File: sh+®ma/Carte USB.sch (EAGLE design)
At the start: 12 parts, among them X2 PN61729-S, X4 87758-0216, X5 PN61729-S, X7 PN61729-S, X8 PN61729-S

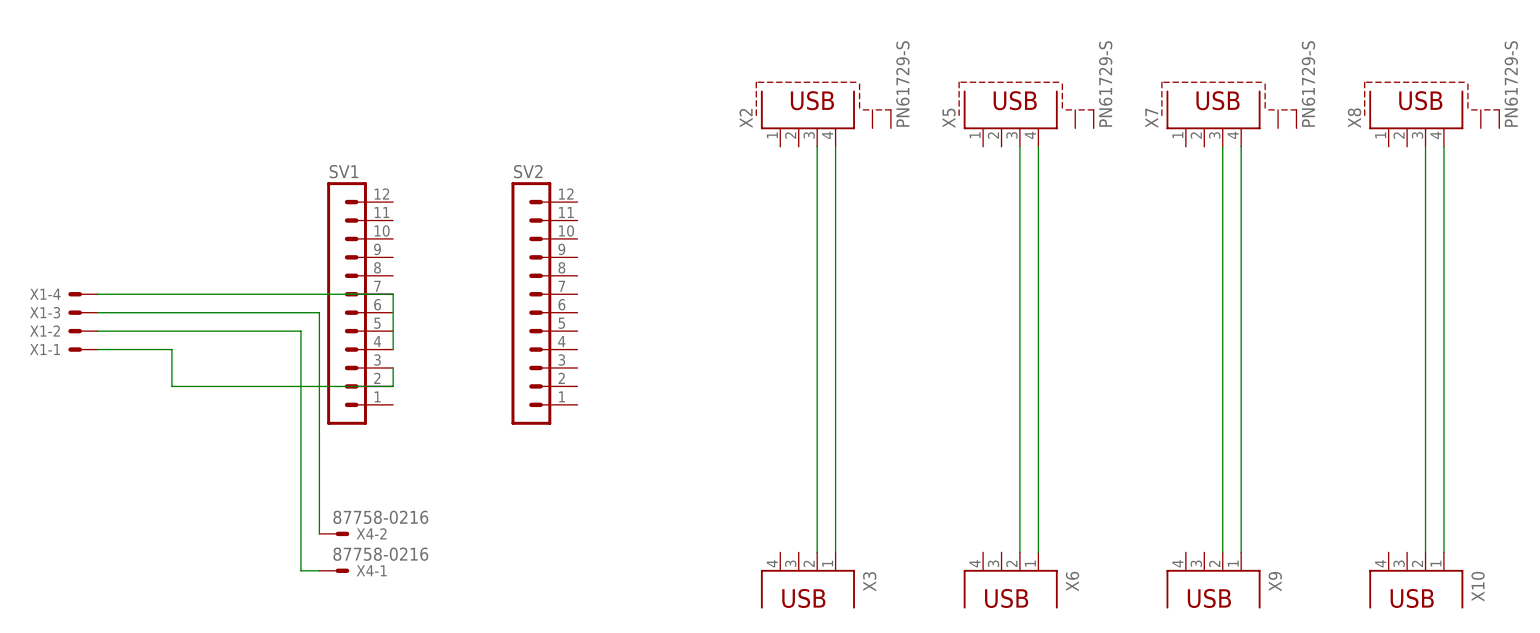
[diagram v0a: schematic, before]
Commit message: typon + plaque fond
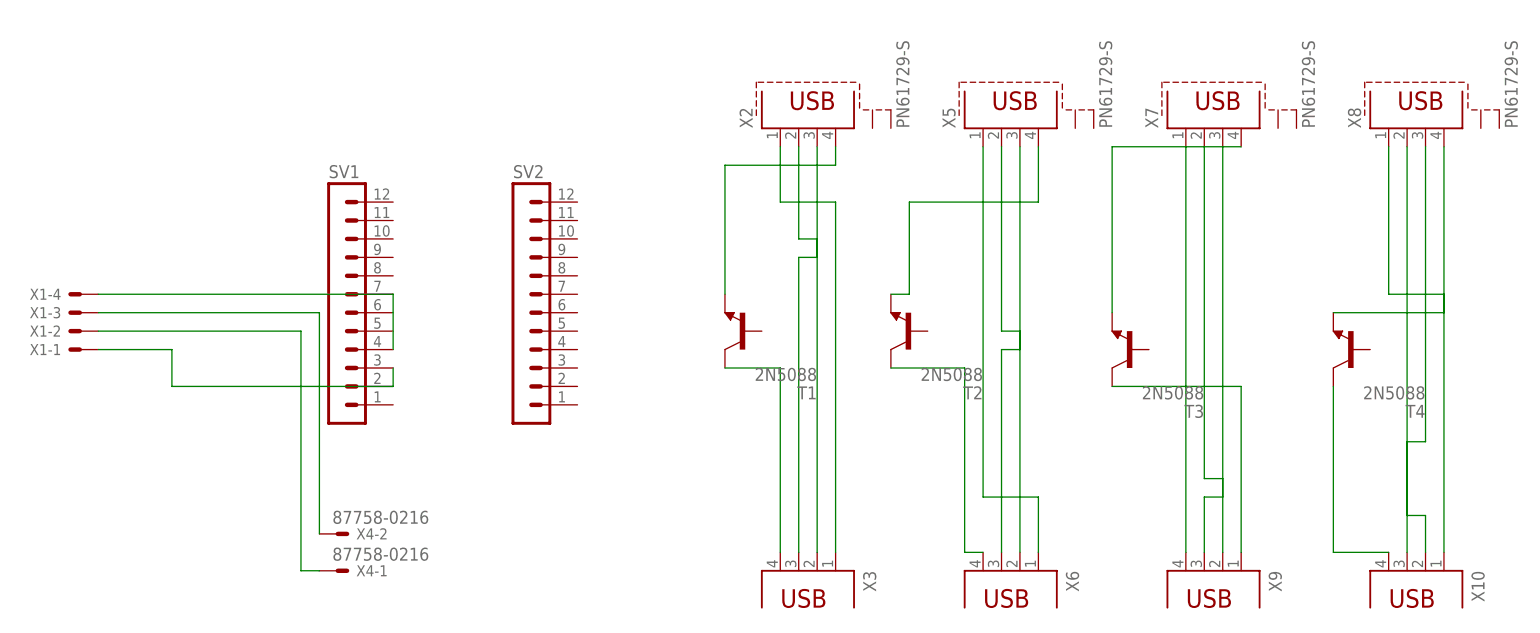
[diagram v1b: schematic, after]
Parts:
- added T1, T2, T3, T4: 2N5088, transistor:2N5088
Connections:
- new net N$14: X7.3, X9.3
- new net N$15: X10.1, X8.1
- new net N$16: X10.2, X8.2
- new net N$17: X10.3, X8.3
- new net N$18: T1.E, X2.4
- new net N$19: T1.C, X3.4
- new net N$20: T2.C, X6.4
- new net N$21: T2.E, X5.4
- new net N$22: T3.E, X7.4
- new net N$23: T3.C, X9.4
- new net N$24: T4.C, X10.4
- new net N$25: T4.E, X8.4
- net N$10: now also X5.2, X6.2; no longer X7.4, X9.1
- net N$11: now also X7.1, X9.1; no longer X10.2, X8.3
- net N$12: now also X7.2, X9.2; no longer X10.1, X8.4
- net N$3: now also X2.1; no longer X2.4
- net N$4: now also X2.2; no longer X2.3
- net N$7: now also X2.3, X3.3; no longer X5.4, X6.1
- net N$8: now also X6.3; no longer X6.2
- net N$9: now also X5.1, X6.1; no longer X7.3, X9.2
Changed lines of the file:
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@@
 <part name="X9" library="con-berg" deviceset="PN87520" device=""/>
 <part name="X10" library="con-berg" deviceset="PN87520" device=""/>
+<part name="T1" library="transistor" deviceset="2N5088" device=""/>
+<part name="T2" library="transistor" deviceset="2N5088" device=""/>
+<part name="T3" library="transistor" deviceset="2N5088" device=""/>
+<part name="T4" library="transistor" deviceset="2N5088" device=""/>
 </parts>
 <sheets>
@@
 <instance part="X9" gate="G$1" x="144.78" y="15.24" rot="R270"/>
 <instance part="X10" gate="G$1" x="172.72" y="15.24" rot="R270"/>
+<instance part="T1" gate="G$1" x="81.28" y="48.26" rot="R180"/>
+<instance part="T2" gate="G$1" x="104.14" y="48.26" rot="R180"/>
+<instance part="T3" gate="G$1" x="134.62" y="45.72" rot="R180"/>
+<instance part="T4" gate="G$1" x="165.1" y="45.72" rot="R180"/>
 </instances>
 <busses>
@@
 <pinref part="X4" gate="-1" pin="S"/>
 <wire x1="20.32" y1="15.24" x2="22.86" y2="15.24" width="0.1524" layer="91"/>
-</segment>
-</net>
-<net name="N$3" class="0">
-<segment>
-<pinref part="X2" gate="G$1" pin="4"/>
-<pinref part="X3" gate="G$1" pin="1"/>
-<wire x1="93.98" y1="73.66" x2="93.98" y2="17.78" width="0.1524" layer="91"/>
-</segment>
-</net>
-<net name="N$4" class="0">
-<segment>
-<pinref part="X2" gate="G$1" pin="3"/>
-<wire x1="91.44" y1="73.66" x2="91.44" y2="17.78" width="0.1524" layer="91"/>
-<pinref part="X3" gate="G$1" pin="2"/>
 </segment>
 </net>
@@
 </segment>
 </net>
+<net name="N$3" class="0">
+<segment>
+<pinref part="X3" gate="G$1" pin="1"/>
+<wire x1="93.98" y1="17.78" x2="93.98" y2="66.04" width="0.1524" layer="91"/>
+<pinref part="X2" gate="G$1" pin="1"/>
+<wire x1="93.98" y1="66.04" x2="86.36" y2="66.04" width="0.1524" layer="91"/>
+<wire x1="86.36" y1="66.04" x2="86.36" y2="73.66" width="0.1524" layer="91"/>
+</segment>
+</net>
+<net name="N$4" class="0">
+<segment>
+<pinref part="X2" gate="G$1" pin="2"/>
+<wire x1="88.9" y1="73.66" x2="88.9" y2="60.96" width="0.1524" layer="91"/>
+<pinref part="X3" gate="G$1" pin="2"/>
+<wire x1="88.9" y1="60.96" x2="91.44" y2="60.96" width="0.1524" layer="91"/>
+<wire x1="91.44" y1="60.96" x2="91.44" y2="17.78" width="0.1524" layer="91"/>
+</segment>
+</net>
 <net name="N$7" class="0">
 <segment>
+<pinref part="X3" gate="G$1" pin="3"/>
+<wire x1="88.9" y1="17.78" x2="88.9" y2="58.42" width="0.1524" layer="91"/>
+<pinref part="X2" gate="G$1" pin="3"/>
+<wire x1="88.9" y1="58.42" x2="91.44" y2="58.42" width="0.1524" layer="91"/>
+<wire x1="91.44" y1="58.42" x2="91.44" y2="73.66" width="0.1524" layer="91"/>
+</segment>
+</net>
+<net name="N$8" class="0">
+<segment>
+<pinref part="X6" gate="G$1" pin="3"/>
+<wire x1="116.84" y1="17.78" x2="116.84" y2="45.72" width="0.1524" layer="91"/>
+<pinref part="X5" gate="G$1" pin="3"/>
+<wire x1="116.84" y1="45.72" x2="119.38" y2="45.72" width="0.1524" layer="91"/>
+<wire x1="119.38" y1="45.72" x2="119.38" y2="73.66" width="0.1524" layer="91"/>
+</segment>
+</net>
+<net name="N$9" class="0">
+<segment>
+<pinref part="X5" gate="G$1" pin="1"/>
+<wire x1="114.3" y1="73.66" x2="114.3" y2="25.4" width="0.1524" layer="91"/>
+<pinref part="X6" gate="G$1" pin="1"/>
+<wire x1="114.3" y1="25.4" x2="121.92" y2="25.4" width="0.1524" layer="91"/>
+<wire x1="121.92" y1="25.4" x2="121.92" y2="17.78" width="0.1524" layer="91"/>
+</segment>
+</net>
+<net name="N$10" class="0">
+<segment>
+<pinref part="X5" gate="G$1" pin="2"/>
+<wire x1="116.84" y1="73.66" x2="116.84" y2="48.26" width="0.1524" layer="91"/>
+<pinref part="X6" gate="G$1" pin="2"/>
+<wire x1="116.84" y1="48.26" x2="119.38" y2="48.26" width="0.1524" layer="91"/>
+<wire x1="119.38" y1="48.26" x2="119.38" y2="17.78" width="0.1524" layer="91"/>
+</segment>
+</net>
+<net name="N$11" class="0">
+<segment>
+<pinref part="X7" gate="G$1" pin="1"/>
+<wire x1="142.24" y1="73.66" x2="142.24" y2="40.64" width="0.1524" layer="91"/>
+<pinref part="X9" gate="G$1" pin="1"/>
+<wire x1="142.24" y1="40.64" x2="149.86" y2="40.64" width="0.1524" layer="91"/>
+<wire x1="149.86" y1="40.64" x2="149.86" y2="17.78" width="0.1524" layer="91"/>
+</segment>
+</net>
+<net name="N$12" class="0">
+<segment>
+<pinref part="X7" gate="G$1" pin="2"/>
+<wire x1="144.78" y1="73.66" x2="144.78" y2="27.94" width="0.1524" layer="91"/>
+<pinref part="X9" gate="G$1" pin="2"/>
+<wire x1="144.78" y1="27.94" x2="147.32" y2="27.94" width="0.1524" layer="91"/>
+<wire x1="147.32" y1="27.94" x2="147.32" y2="17.78" width="0.1524" layer="91"/>
+</segment>
+</net>
+<net name="N$14" class="0">
+<segment>
+<pinref part="X9" gate="G$1" pin="3"/>
+<wire x1="144.78" y1="17.78" x2="144.78" y2="25.4" width="0.1524" layer="91"/>
+<pinref part="X7" gate="G$1" pin="3"/>
+<wire x1="144.78" y1="25.4" x2="147.32" y2="25.4" width="0.1524" layer="91"/>
+<wire x1="147.32" y1="25.4" x2="147.32" y2="73.66" width="0.1524" layer="91"/>
+</segment>
+</net>
+<net name="N$15" class="0">
+<segment>
+<pinref part="X10" gate="G$1" pin="1"/>
+<wire x1="177.8" y1="17.78" x2="177.8" y2="53.34" width="0.1524" layer="91"/>
+<pinref part="X8" gate="G$1" pin="1"/>
+<wire x1="177.8" y1="53.34" x2="170.18" y2="53.34" width="0.1524" layer="91"/>
+<wire x1="170.18" y1="53.34" x2="170.18" y2="73.66" width="0.1524" layer="91"/>
+</segment>
+</net>
+<net name="N$16" class="0">
+<segment>
+<pinref part="X8" gate="G$1" pin="2"/>
+<wire x1="172.72" y1="73.66" x2="172.72" y2="22.86" width="0.1524" layer="91"/>
+<pinref part="X10" gate="G$1" pin="2"/>
+<wire x1="172.72" y1="22.86" x2="175.26" y2="22.86" width="0.1524" layer="91"/>
+<wire x1="175.26" y1="22.86" x2="175.26" y2="17.78" width="0.1524" layer="91"/>
+</segment>
+</net>
+<net name="N$17" class="0">
+<segment>
+<pinref part="X8" gate="G$1" pin="3"/>
+<wire x1="175.26" y1="73.66" x2="175.26" y2="33.02" width="0.1524" layer="91"/>
+<pinref part="X10" gate="G$1" pin="3"/>
+<wire x1="175.26" y1="33.02" x2="172.72" y2="33.02" width="0.1524" layer="91"/>
+<wire x1="172.72" y1="33.02" x2="172.72" y2="17.78" width="0.1524" layer="91"/>
+</segment>
+</net>
+<net name="N$18" class="0">
+<segment>
+<pinref part="X2" gate="G$1" pin="4"/>
+<wire x1="93.98" y1="73.66" x2="93.98" y2="71.12" width="0.1524" layer="91"/>
+<pinref part="T1" gate="G$1" pin="E"/>
+<wire x1="93.98" y1="71.12" x2="78.74" y2="71.12" width="0.1524" layer="91"/>
+<wire x1="78.74" y1="71.12" x2="78.74" y2="53.34" width="0.1524" layer="91"/>
+</segment>
+</net>
+<net name="N$19" class="0">
+<segment>
+<pinref part="T1" gate="G$1" pin="C"/>
+<pinref part="X3" gate="G$1" pin="4"/>
+<wire x1="78.74" y1="43.18" x2="86.36" y2="43.18" width="0.1524" layer="91"/>
+<wire x1="86.36" y1="43.18" x2="86.36" y2="17.78" width="0.1524" layer="91"/>
+</segment>
+</net>
+<net name="N$20" class="0">
+<segment>
+<pinref part="T2" gate="G$1" pin="C"/>
+<wire x1="101.6" y1="43.18" x2="111.76" y2="43.18" width="0.1524" layer="91"/>
+<wire x1="111.76" y1="43.18" x2="111.76" y2="17.78" width="0.1524" layer="91"/>
+<pinref part="X6" gate="G$1" pin="4"/>
+<wire x1="111.76" y1="17.78" x2="114.3" y2="17.78" width="0.1524" layer="91"/>
+</segment>
+</net>
+<net name="N$21" class="0">
+<segment>
+<pinref part="T2" gate="G$1" pin="E"/>
+<wire x1="101.6" y1="53.34" x2="104.14" y2="53.34" width="0.1524" layer="91"/>
+<wire x1="104.14" y1="53.34" x2="104.14" y2="66.04" width="0.1524" layer="91"/>
 <pinref part="X5" gate="G$1" pin="4"/>
-<pinref part="X6" gate="G$1" pin="1"/>
-<wire x1="121.92" y1="73.66" x2="121.92" y2="17.78" width="0.1524" layer="91"/>
-</segment>
-</net>
-<net name="N$8" class="0">
-<segment>
-<pinref part="X5" gate="G$1" pin="3"/>
-<wire x1="119.38" y1="73.66" x2="119.38" y2="17.78" width="0.1524" layer="91"/>
-<pinref part="X6" gate="G$1" pin="2"/>
-</segment>
-</net>
-<net name="N$9" class="0">
-<segment>
-<pinref part="X7" gate="G$1" pin="3"/>
-<pinref part="X9" gate="G$1" pin="2"/>
-<wire x1="147.32" y1="73.66" x2="147.32" y2="17.78" width="0.1524" layer="91"/>
-</segment>
-</net>
-<net name="N$10" class="0">
-<segment>
-<pinref part="X9" gate="G$1" pin="1"/>
+<wire x1="104.14" y1="66.04" x2="121.92" y2="66.04" width="0.1524" layer="91"/>
+<wire x1="121.92" y1="66.04" x2="121.92" y2="73.66" width="0.1524" layer="91"/>
+</segment>
+</net>
+<net name="N$22" class="0">
+<segment>
 <pinref part="X7" gate="G$1" pin="4"/>
-<wire x1="149.86" y1="17.78" x2="149.86" y2="73.66" width="0.1524" layer="91"/>
-</segment>
-</net>
-<net name="N$11" class="0">
-<segment>
-<pinref part="X8" gate="G$1" pin="3"/>
-<pinref part="X10" gate="G$1" pin="2"/>
-<wire x1="175.26" y1="73.66" x2="175.26" y2="17.78" width="0.1524" layer="91"/>
-</segment>
-</net>
-<net name="N$12" class="0">
-<segment>
-<pinref part="X10" gate="G$1" pin="1"/>
+<pinref part="T3" gate="G$1" pin="E"/>
+<wire x1="149.86" y1="73.66" x2="132.08" y2="73.66" width="0.1524" layer="91"/>
+<wire x1="132.08" y1="73.66" x2="132.08" y2="50.8" width="0.1524" layer="91"/>
+</segment>
+</net>
+<net name="N$23" class="0">
+<segment>
+<pinref part="T3" gate="G$1" pin="C"/>
+<pinref part="X9" gate="G$1" pin="4"/>
+<wire x1="132.08" y1="40.64" x2="142.24" y2="40.64" width="0.1524" layer="91"/>
+<wire x1="142.24" y1="40.64" x2="142.24" y2="17.78" width="0.1524" layer="91"/>
+</segment>
+</net>
+<net name="N$24" class="0">
+<segment>
+<pinref part="X10" gate="G$1" pin="4"/>
+<pinref part="T4" gate="G$1" pin="C"/>
+<wire x1="170.18" y1="17.78" x2="162.56" y2="17.78" width="0.1524" layer="91"/>
+<wire x1="162.56" y1="17.78" x2="162.56" y2="40.64" width="0.1524" layer="91"/>
+</segment>
+</net>
+<net name="N$25" class="0">
+<segment>
+<pinref part="T4" gate="G$1" pin="E"/>
 <pinref part="X8" gate="G$1" pin="4"/>
-<wire x1="177.8" y1="17.78" x2="177.8" y2="73.66" width="0.1524" layer="91"/>
-</segment>
-</net>
+<wire x1="162.56" y1="50.8" x2="177.8" y2="50.8" width="0.1524" layer="91"/>
+<wire x1="177.8" y1="50.8" x2="177.8" y2="73.66" width="0.1524" layer="91"/>
+</segment>
+</net>
